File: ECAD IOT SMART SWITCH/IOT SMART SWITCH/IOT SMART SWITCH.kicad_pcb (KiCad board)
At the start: 2 copper layers, 42 parts, among them J1 Conn_02x02_Odd_Even, J2 Conn_02x02_Odd_Even, J3 Conn_02x02_Odd_Even, J4 Conn_01x16, J5 Conn_01x16, J6 Conn_02x02_Odd_Even, J7 Conn_02x02_Odd_Even, K1 SLA-12VDC-SL-C, Q1 BS170, T1 VC_10_1_18, T2 AC-1020, U1 4N25, U2 LM317_TO39, U3 LM317_TO39

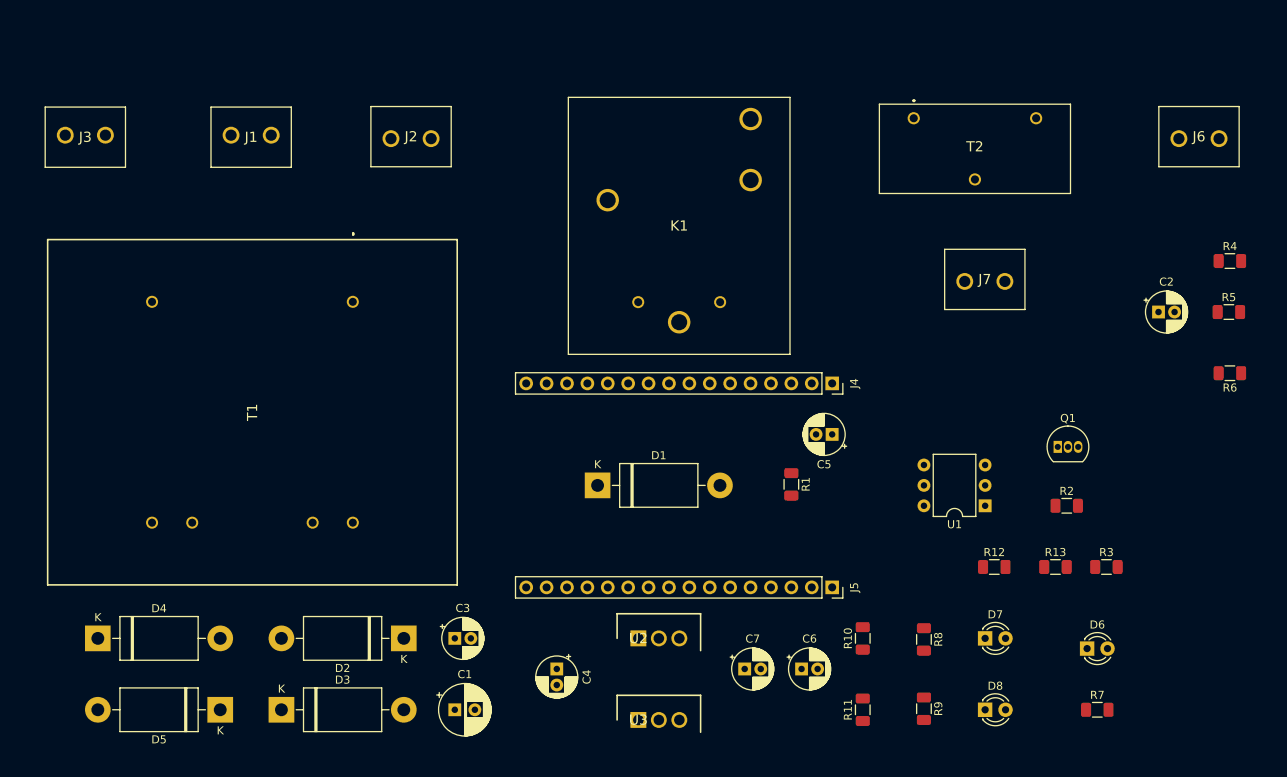
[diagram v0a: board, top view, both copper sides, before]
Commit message: Is fridge running
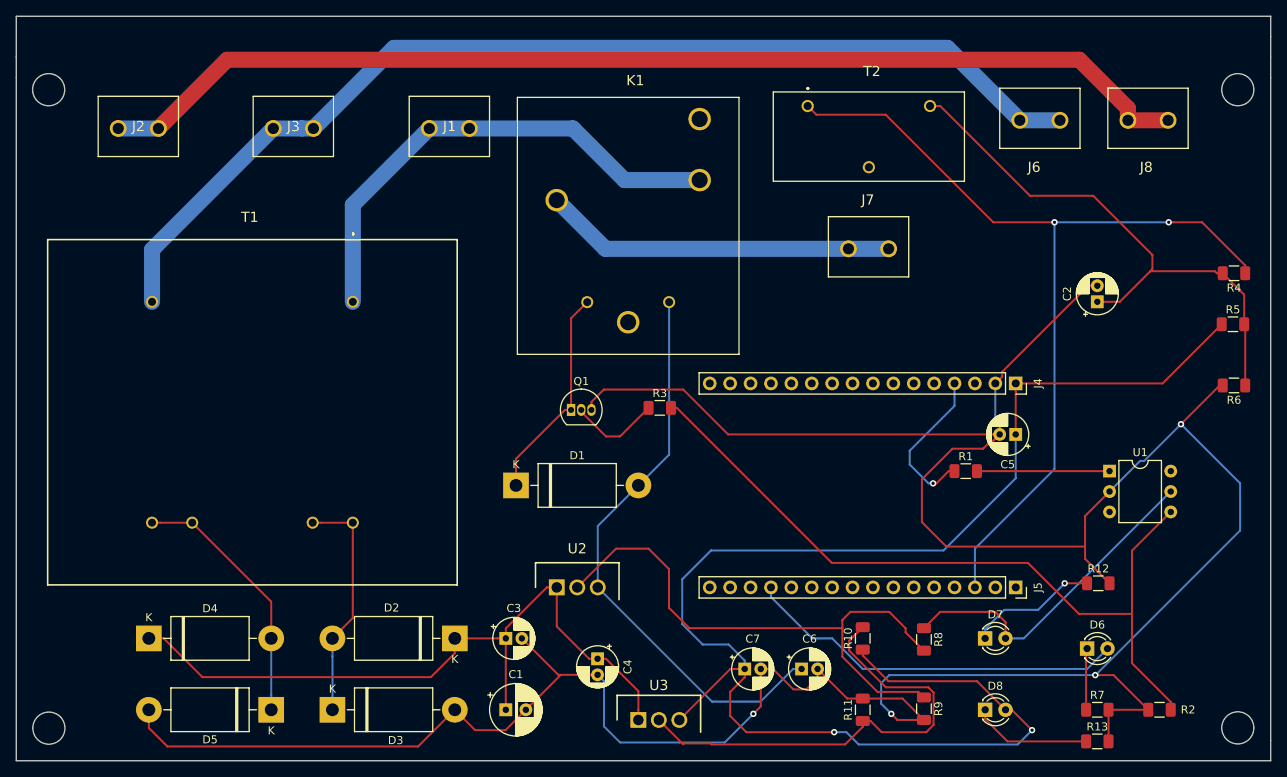
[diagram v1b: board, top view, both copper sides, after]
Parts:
- added J8: KF301-2P, KF3012P, F.Cu at (204.5, 44.7)
- J1, J2, J3, J6, J7: value Conn_02x02_Odd_Even -> KF301-2P; footprint KF301-2P:KF3012P -> KF3012P
- moved Q1 60.8 mm to (135.1, 80.8)
- moved R3 59.0 mm to (146.2, 80.5)
- moved J2 34.0 mm to (78.7, 45.7)
- moved R2 27.9 mm to (208.4, 118.1), turned to 180 degrees
- moved C5 22.9 mm to (190.5, 83.8)
- moved J4 22.9 mm to (190.5, 77.5)
- moved J5 22.9 mm to (190.5, 102.9)
- moved R13 22.3 mm to (200.7, 122.0)
- moved R1 21.8 mm to (184.3, 88.4), turned to 0 degrees
- moved J3 20.9 mm to (98.0, 45.7), turned to 0 degrees
- moved J6 19.9 mm to (191.0, 44.7)
- moved J1 19.7 mm to (117.5, 45.7), turned to 0 degrees
- moved U1 16.1 mm to (202.2, 88.4), turned to 0 degrees
- moved J7 15.0 mm to (169.7, 60.7)
- moved T2 13.3 mm to (172.2, 46.7)
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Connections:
- J1 pad 1: Net-(J1-Pad1) -> MAINS_L
- J1 pad 2: Net-(J1-Pad2) -> MAINS_L
- J2 pad 1: Net-(J2-Pad1) -> Earth
- J2 pad 2: MAINS_L -> Earth
- J3 pad 1: Net-(J3-Pad1) -> MAINS_N
- J6 pad 2: Net-(J6-Pad2) -> MAINS_N
- J7 pad 2: Net-(J7-Pad2) -> Net-(J7-Pad1)
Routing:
- net GNDPWR: track 0.00 -> 377.7 mm, vias 0 -> 4
- net 3V3_DC: track 0.00 -> 186.4 mm, vias 0 -> 2
- net Earth: track 0.00 -> 138.3 mm
- net MAINS_N: track 0.00 -> 133.7 mm
- net 12V_DC: track 0.00 -> 113.9 mm
- net CT_ADC: track 0.00 -> 113.3 mm, vias 0 -> 2
- net Net-(R2-Pad1): track 0.00 -> 96.7 mm
- net 16V_DC: track 0.00 -> 90.1 mm
- net Net-(R8-Pad2): track 0.00 -> 71.7 mm
- net Net-(C2-Pad1): track 0.00 -> 69.9 mm
- net MAINS_L: track 0.00 -> 61.9 mm
- net Net-(R10-Pad2): track 0.00 -> 58.6 mm
- net Net-(D6-Pad2): track 0.00 -> 47.9 mm
- net Net-(J7-Pad1): track 0.00 -> 43.8 mm
- net -18V_AC: track 0.00 -> 32.4 mm
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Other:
- board outline added: 156.2 x 92.7 mm
- net class HV_NET added: clearance 4, trace_width 2, via_dia 0.8, via_drill 0.4
